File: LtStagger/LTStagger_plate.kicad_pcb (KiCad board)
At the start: 2 copper layers, 155 x 112 mm, 22 parts, among them K0 K00, K1 K01, K10 K10, K11 K11, K12 K12, K2 K02, K20 K20, K21 K21, K22 K22, K30 K30, K31 K31, K32 K32, K33 K33, K40 K40, K41 K41, K42 K42, K43 K43, K50 K50, K51 K51, K53 K53, SW1 Rotary_Encoder_Switch

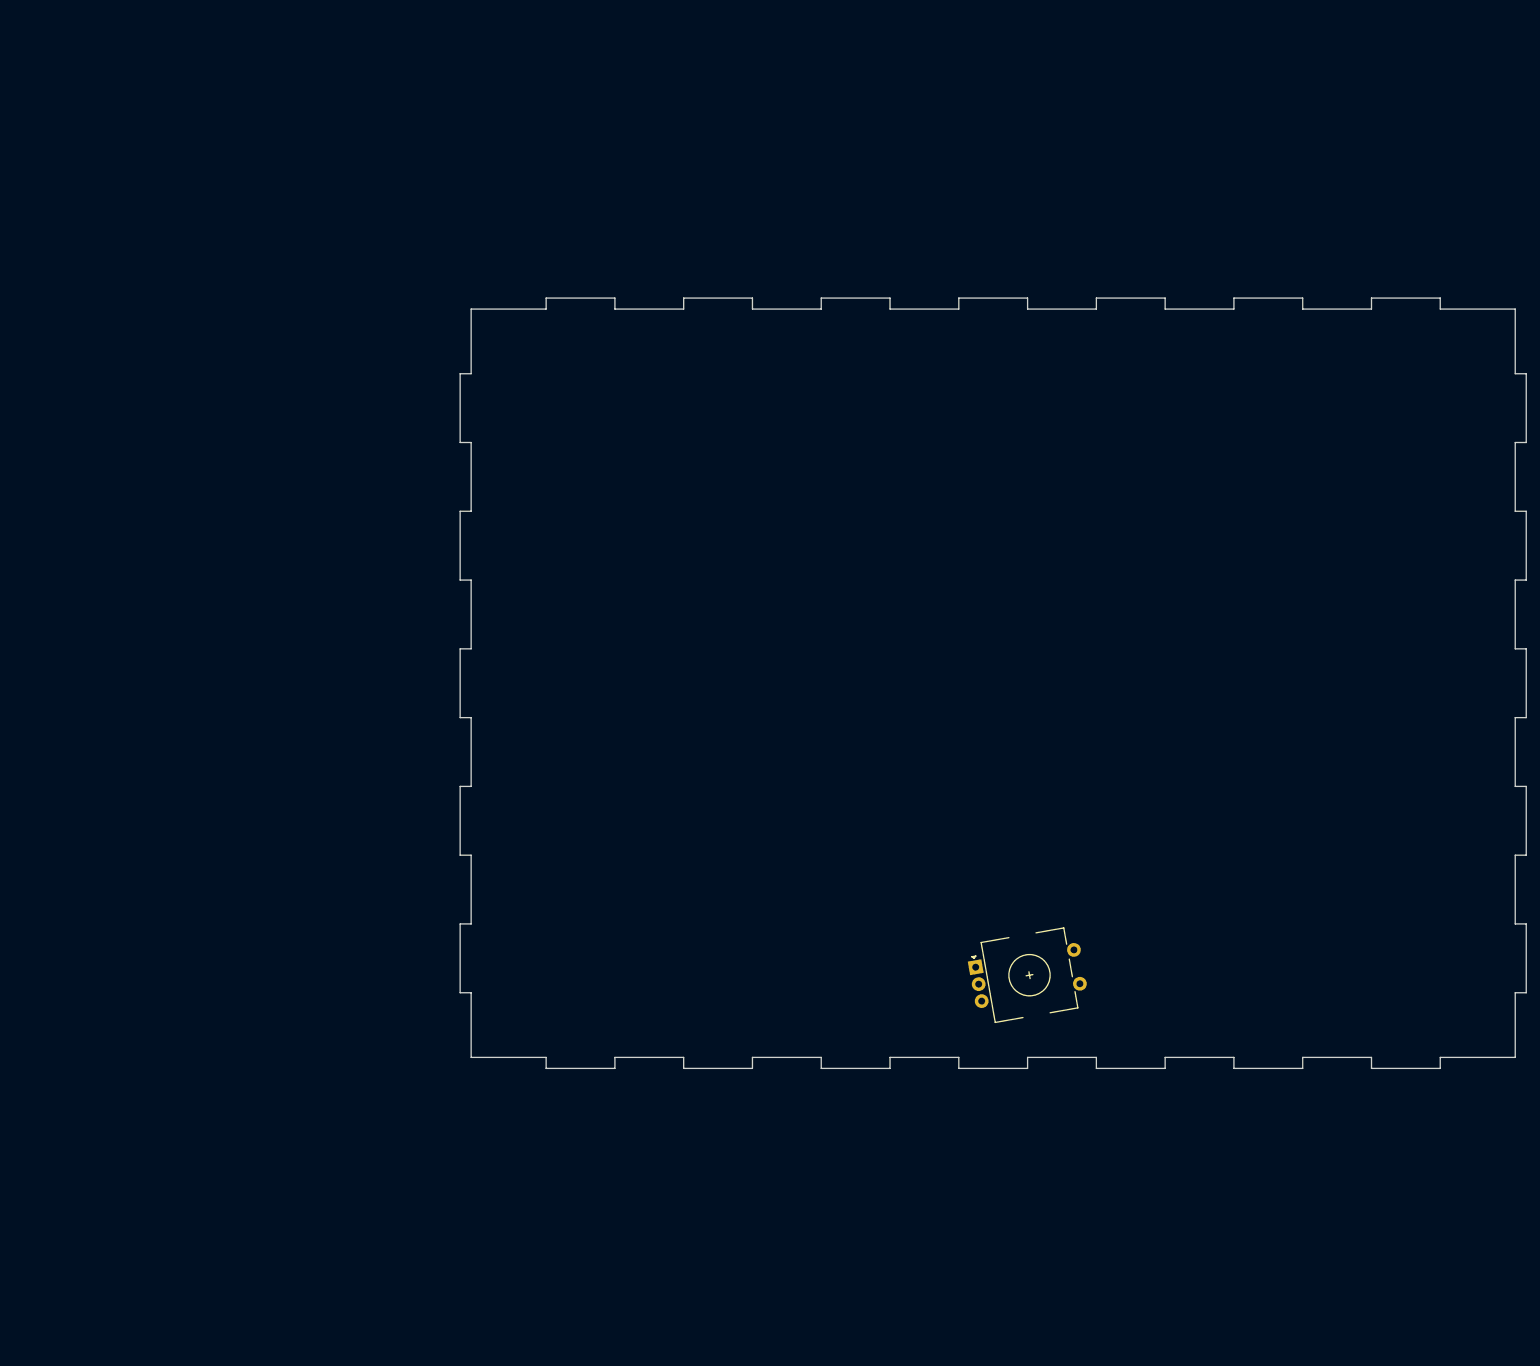
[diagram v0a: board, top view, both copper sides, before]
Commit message: about to give an angle and dog bones
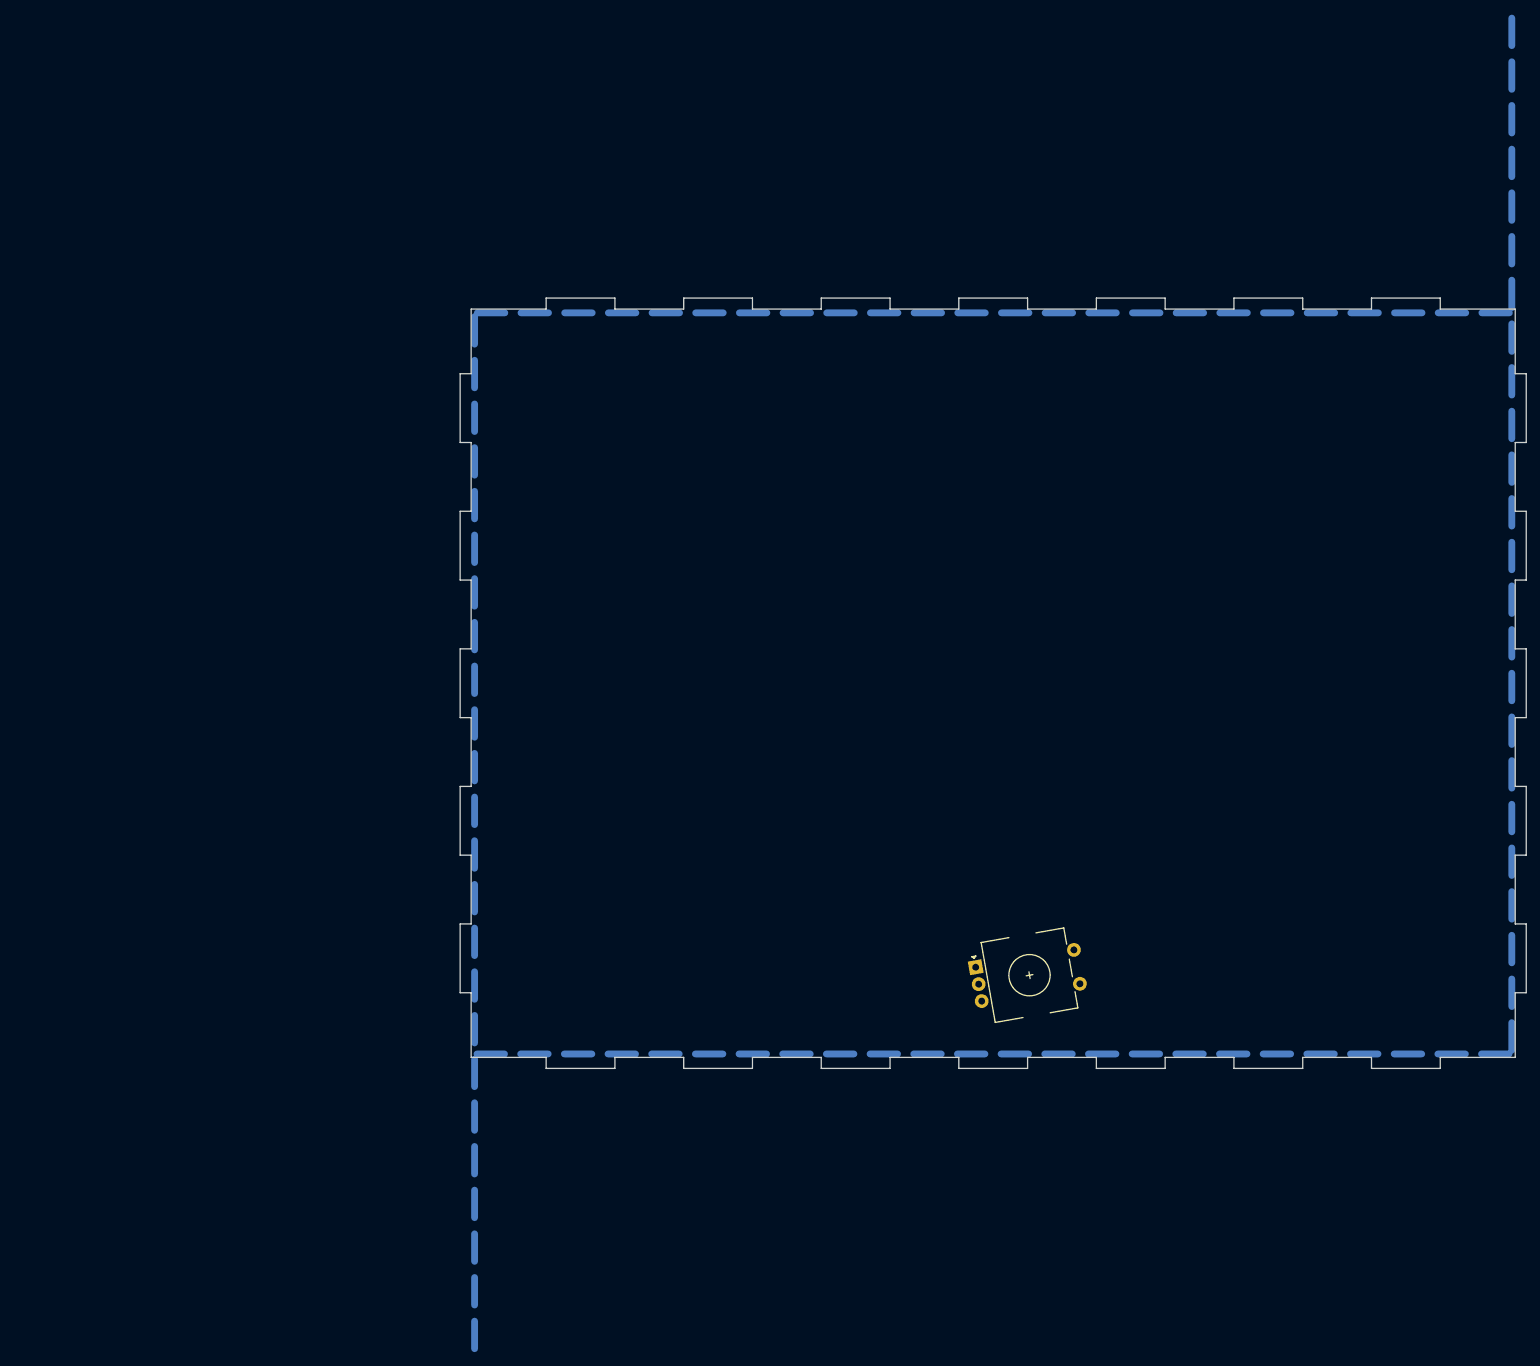
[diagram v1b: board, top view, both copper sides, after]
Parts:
- added REF**: Long_Pad_single_sided, Digi:Long_Pad_single_sided, B.Cu at (64.4, 45.5)
- added REF**: Long_Pad_single_sided, Digi:Long_Pad_single_sided, B.Cu at (215.2, 148.2)
- added REF**: Long_Pad_single_sided, Digi:Long_Pad_single_sided, B.Cu at (66.8, 150.7)
- added REF**: Long_Pad_single_sided, Digi:Long_Pad_single_sided, B.Cu at (66.8, 43.0)
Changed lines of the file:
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@@
     (tracks 0)
     (zones 0)
-    (modules 22)
+    (modules 26)
     (nets 6)
   )
   (page A4)
   (layers
-    (0 F.Cu signal hide)
-    (31 B.Cu signal hide)
+    (0 F.Cu signal)
+    (31 B.Cu signal)
     (32 B.Adhes user hide)
     (33 F.Adhes user hide)
@@
     (diff_pair_gap 0.25)
   )
+  (module Digi:Long_Pad_single_sided (layer B.Cu)
+    (at 64.4 45.5 270)
+    (fp_text reference REF** (at 0 -0.5 90) (layer B.SilkS)
+      (effects (font (size 1 1) (thickness 0.15)) (justify mirror))
+    )
+    (fp_text value Long_Pad_single_sided (at 0 0.5 90) (layer B.Fab)
+      (effects (font (size 1 1) (thickness 0.15)) (justify mirror))
+    )
+    (pad 1 smd oval (at 0 0 270) (size 5 1) (layers B.Cu B.Paste B.Mask))
+    (pad 1 smd oval (at 6.35 0 270) (size 5 1) (layers B.Cu B.Paste B.Mask))
+    (pad 1 smd oval (at 12.7 0 270) (size 5 1) (layers B.Cu B.Paste B.Mask))
+    (pad 1 smd oval (at 19.05 0 270) (size 5 1) (layers B.Cu B.Paste B.Mask))
+    (pad 1 smd oval (at 25.4 0 270) (size 5 1) (layers B.Cu B.Paste B.Mask))
+    (pad 1 smd oval (at 31.75 0 270) (size 5 1) (layers B.Cu B.Paste B.Mask))
+    (pad 1 smd oval (at 38.1 0 270) (size 5 1) (layers B.Cu B.Paste B.Mask))
+    (pad 1 smd oval (at 44.45 0 270) (size 5 1) (layers B.Cu B.Paste B.Mask))
+    (pad 1 smd oval (at 50.8 0 270) (size 5 1) (layers B.Cu B.Paste B.Mask))
+    (pad 1 smd oval (at 57.15 0 270) (size 5 1) (layers B.Cu B.Paste B.Mask))
+    (pad 1 smd oval (at 63.5 0 270) (size 5 1) (layers B.Cu B.Paste B.Mask))
+    (pad 1 smd oval (at 69.85 0 270) (size 5 1) (layers B.Cu B.Paste B.Mask))
+    (pad 1 smd oval (at 76.2 0 270) (size 5 1) (layers B.Cu B.Paste B.Mask))
+    (pad 1 smd oval (at 82.55 0 270) (size 5 1) (layers B.Cu B.Paste B.Mask))
+    (pad 1 smd oval (at 88.9 0 270) (size 5 1) (layers B.Cu B.Paste B.Mask))
+    (pad 1 smd oval (at 95.25 0 270) (size 5 1) (layers B.Cu B.Paste B.Mask))
+    (pad 1 smd oval (at 101.6 0 270) (size 5 1) (layers B.Cu B.Paste B.Mask))
+    (pad 1 smd oval (at 107.95 0 270) (size 5 1) (layers B.Cu B.Paste B.Mask))
+    (pad 1 smd oval (at 114.3 0 270) (size 5 1) (layers B.Cu B.Paste B.Mask))
+    (pad 1 smd oval (at 120.65 0 270) (size 5 1) (layers B.Cu B.Paste B.Mask))
+    (pad 1 smd oval (at 127 0 270) (size 5 1) (layers B.Cu B.Paste B.Mask))
+    (pad 1 smd oval (at 133.35 0 270) (size 5 1) (layers B.Cu B.Paste B.Mask))
+    (pad 1 smd oval (at 139.7 0 270) (size 5 1) (layers B.Cu B.Paste B.Mask))
+    (pad 1 smd oval (at 146.05 0 270) (size 5 1) (layers B.Cu B.Paste B.Mask))
+  )
+  (module Digi:Long_Pad_single_sided (layer B.Cu)
+    (at 215.2 148.15 90)
+    (fp_text reference REF** (at 0 -0.5 90) (layer B.SilkS)
+      (effects (font (size 1 1) (thickness 0.15)) (justify mirror))
+    )
+    (fp_text value Long_Pad_single_sided (at 0 0.5 90) (layer B.Fab)
+      (effects (font (size 1 1) (thickness 0.15)) (justify mirror))
+    )
+    (pad 1 smd oval (at 0 0 90) (size 5 1) (layers B.Cu B.Paste B.Mask))
+    (pad 1 smd oval (at 6.35 0 90) (size 5 1) (layers B.Cu B.Paste B.Mask))
+    (pad 1 smd oval (at 12.7 0 90) (size 5 1) (layers B.Cu B.Paste B.Mask))
+    (pad 1 smd oval (at 19.05 0 90) (size 5 1) (layers B.Cu B.Paste B.Mask))
+    (pad 1 smd oval (at 25.4 0 90) (size 5 1) (layers B.Cu B.Paste B.Mask))
+    (pad 1 smd oval (at 31.75 0 90) (size 5 1) (layers B.Cu B.Paste B.Mask))
+    (pad 1 smd oval (at 38.1 0 90) (size 5 1) (layers B.Cu B.Paste B.Mask))
+    (pad 1 smd oval (at 44.45 0 90) (size 5 1) (layers B.Cu B.Paste B.Mask))
+    (pad 1 smd oval (at 50.8 0 90) (size 5 1) (layers B.Cu B.Paste B.Mask))
+    (pad 1 smd oval (at 57.15 0 90) (size 5 1) (layers B.Cu B.Paste B.Mask))
+    (pad 1 smd oval (at 63.5 0 90) (size 5 1) (layers B.Cu B.Paste B.Mask))
+    (pad 1 smd oval (at 69.85 0 90) (size 5 1) (layers B.Cu B.Paste B.Mask))
+    (pad 1 smd oval (at 76.2 0 90) (size 5 1) (layers B.Cu B.Paste B.Mask))
+    (pad 1 smd oval (at 82.55 0 90) (size 5 1) (layers B.Cu B.Paste B.Mask))
+    (pad 1 smd oval (at 88.9 0 90) (size 5 1) (layers B.Cu B.Paste B.Mask))
+    (pad 1 smd oval (at 95.25 0 90) (size 5 1) (layers B.Cu B.Paste B.Mask))
+    (pad 1 smd oval (at 101.6 0 90) (size 5 1) (layers B.Cu B.Paste B.Mask))
+    (pad 1 smd oval (at 107.95 0 90) (size 5 1) (layers B.Cu B.Paste B.Mask))
+    (pad 1 smd oval (at 114.3 0 90) (size 5 1) (layers B.Cu B.Paste B.Mask))
+    (pad 1 smd oval (at 120.65 0 90) (size 5 1) (layers B.Cu B.Paste B.Mask))
+    (pad 1 smd oval (at 127 0 90) (size 5 1) (layers B.Cu B.Paste B.Mask))
+    (pad 1 smd oval (at 133.35 0 90) (size 5 1) (layers B.Cu B.Paste B.Mask))
+    (pad 1 smd oval (at 139.7 0 90) (size 5 1) (layers B.Cu B.Paste B.Mask))
+    (pad 1 smd oval (at 146.05 0 90) (size 5 1) (layers B.Cu B.Paste B.Mask))
+  )
+  (module Digi:Long_Pad_single_sided (layer B.Cu)
+    (at 66.75 150.7)
+    (fp_text reference REF** (at 0 -0.5) (layer B.SilkS)
+      (effects (font (size 1 1) (thickness 0.15)) (justify mirror))
+    )
+    (fp_text value Long_Pad_single_sided (at 0 0.5) (layer B.Fab)
+      (effects (font (size 1 1) (thickness 0.15)) (justify mirror))
+    )
+    (pad 1 smd oval (at 0 0) (size 5 1) (layers B.Cu B.Paste B.Mask))
+    (pad 1 smd oval (at 6.35 0) (size 5 1) (layers B.Cu B.Paste B.Mask))
+    (pad 1 smd oval (at 12.7 0) (size 5 1) (layers B.Cu B.Paste B.Mask))
+    (pad 1 smd oval (at 19.05 0) (size 5 1) (layers B.Cu B.Paste B.Mask))
+    (pad 1 smd oval (at 25.4 0) (size 5 1) (layers B.Cu B.Paste B.Mask))
+    (pad 1 smd oval (at 31.75 0) (size 5 1) (layers B.Cu B.Paste B.Mask))
+    (pad 1 smd oval (at 38.1 0) (size 5 1) (layers B.Cu B.Paste B.Mask))
+    (pad 1 smd oval (at 44.45 0) (size 5 1) (layers B.Cu B.Paste B.Mask))
+    (pad 1 smd oval (at 50.8 0) (size 5 1) (layers B.Cu B.Paste B.Mask))
+    (pad 1 smd oval (at 57.15 0) (size 5 1) (layers B.Cu B.Paste B.Mask))
+    (pad 1 smd oval (at 63.5 0) (size 5 1) (layers B.Cu B.Paste B.Mask))
+    (pad 1 smd oval (at 69.85 0) (size 5 1) (layers B.Cu B.Paste B.Mask))
+    (pad 1 smd oval (at 76.2 0) (size 5 1) (layers B.Cu B.Paste B.Mask))
+    (pad 1 smd oval (at 82.55 0) (size 5 1) (layers B.Cu B.Paste B.Mask))
+    (pad 1 smd oval (at 88.9 0) (size 5 1) (layers B.Cu B.Paste B.Mask))
+    (pad 1 smd oval (at 95.25 0) (size 5 1) (layers B.Cu B.Paste B.Mask))
+    (pad 1 smd oval (at 101.6 0) (size 5 1) (layers B.Cu B.Paste B.Mask))
+    (pad 1 smd oval (at 107.95 0) (size 5 1) (layers B.Cu B.Paste B.Mask))
+    (pad 1 smd oval (at 114.3 0) (size 5 1) (layers B.Cu B.Paste B.Mask))
+    (pad 1 smd oval (at 120.65 0) (size 5 1) (layers B.Cu B.Paste B.Mask))
+    (pad 1 smd oval (at 127 0) (size 5 1) (layers B.Cu B.Paste B.Mask))
+    (pad 1 smd oval (at 133.35 0) (size 5 1) (layers B.Cu B.Paste B.Mask))
+    (pad 1 smd oval (at 139.7 0) (size 5 1) (layers B.Cu B.Paste B.Mask))
+    (pad 1 smd oval (at 146.05 0) (size 5 1) (layers B.Cu B.Paste B.Mask))
+  )
+  (module Digi:Long_Pad_single_sided (layer B.Cu)
+    (at 66.8 42.95)
+    (fp_text reference REF** (at 0 -0.5) (layer B.SilkS)
+      (effects (font (size 1 1) (thickness 0.15)) (justify mirror))
+    )
+    (fp_text value Long_Pad_single_sided (at 0 0.5) (layer B.Fab)
+      (effects (font (size 1 1) (thickness 0.15)) (justify mirror))
+    )
+    (pad 1 smd oval (at 146.05 0) (size 5 1) (layers B.Cu B.Paste B.Mask))
+    (pad 1 smd oval (at 139.7 0) (size 5 1) (layers B.Cu B.Paste B.Mask))
+    (pad 1 smd oval (at 133.35 0) (size 5 1) (layers B.Cu B.Paste B.Mask))
+    (pad 1 smd oval (at 127 0) (size 5 1) (layers B.Cu B.Paste B.Mask))
+    (pad 1 smd oval (at 120.65 0) (size 5 1) (layers B.Cu B.Paste B.Mask))
+    (pad 1 smd oval (at 114.3 0) (size 5 1) (layers B.Cu B.Paste B.Mask))
+    (pad 1 smd oval (at 107.95 0) (size 5 1) (layers B.Cu B.Paste B.Mask))
+    (pad 1 smd oval (at 101.6 0) (size 5 1) (layers B.Cu B.Paste B.Mask))
+    (pad 1 smd oval (at 95.25 0) (size 5 1) (layers B.Cu B.Paste B.Mask))
+    (pad 1 smd oval (at 88.9 0) (size 5 1) (layers B.Cu B.Paste B.Mask))
+    (pad 1 smd oval (at 82.55 0) (size 5 1) (layers B.Cu B.Paste B.Mask))
+    (pad 1 smd oval (at 76.2 0) (size 5 1) (layers B.Cu B.Paste B.Mask))
+    (pad 1 smd oval (at 69.85 0) (size 5 1) (layers B.Cu B.Paste B.Mask))
+    (pad 1 smd oval (at 63.5 0) (size 5 1) (layers B.Cu B.Paste B.Mask))
+    (pad 1 smd oval (at 57.15 0) (size 5 1) (layers B.Cu B.Paste B.Mask))
+    (pad 1 smd oval (at 50.8 0) (size 5 1) (layers B.Cu B.Paste B.Mask))
+    (pad 1 smd oval (at 44.45 0) (size 5 1) (layers B.Cu B.Paste B.Mask))
+    (pad 1 smd oval (at 38.1 0) (size 5 1) (layers B.Cu B.Paste B.Mask))
+    (pad 1 smd oval (at 31.75 0) (size 5 1) (layers B.Cu B.Paste B.Mask))
+    (pad 1 smd oval (at 25.4 0) (size 5 1) (layers B.Cu B.Paste B.Mask))
+    (pad 1 smd oval (at 19.05 0) (size 5 1) (layers B.Cu B.Paste B.Mask))
+    (pad 1 smd oval (at 12.7 0) (size 5 1) (layers B.Cu B.Paste B.Mask))
+    (pad 1 smd oval (at 6.35 0) (size 5 1) (layers B.Cu B.Paste B.Mask))
+    (pad 1 smd oval (at 0 0) (size 5 1) (layers B.Cu B.Paste B.Mask))
+  )
   (module Digi:Plate-1u locked (layer F.Cu)
